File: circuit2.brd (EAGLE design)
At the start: 85.1 x 100 mm, 16 parts, among them IC1 ATMEGA328-20P, IC2 786TV

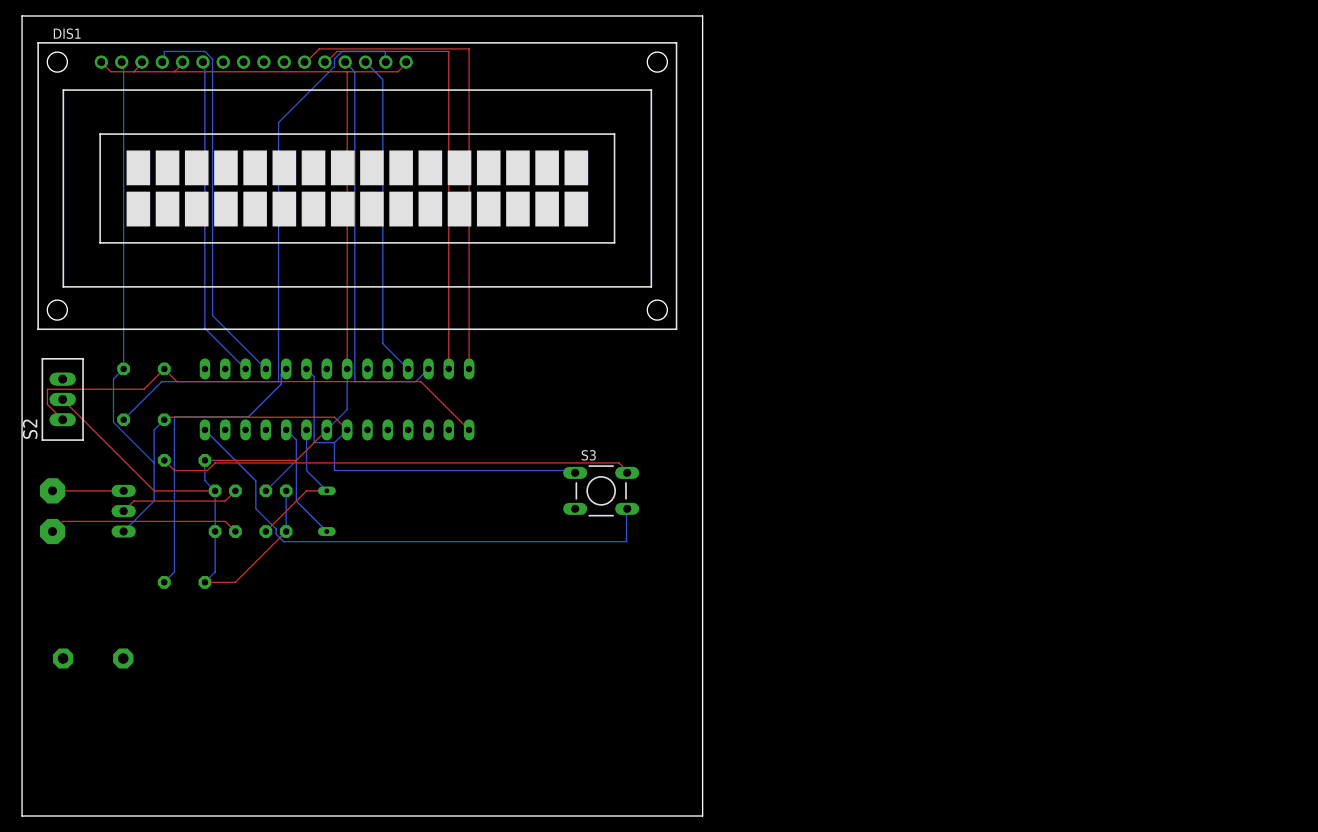
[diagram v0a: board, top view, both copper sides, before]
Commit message: Add files via upload
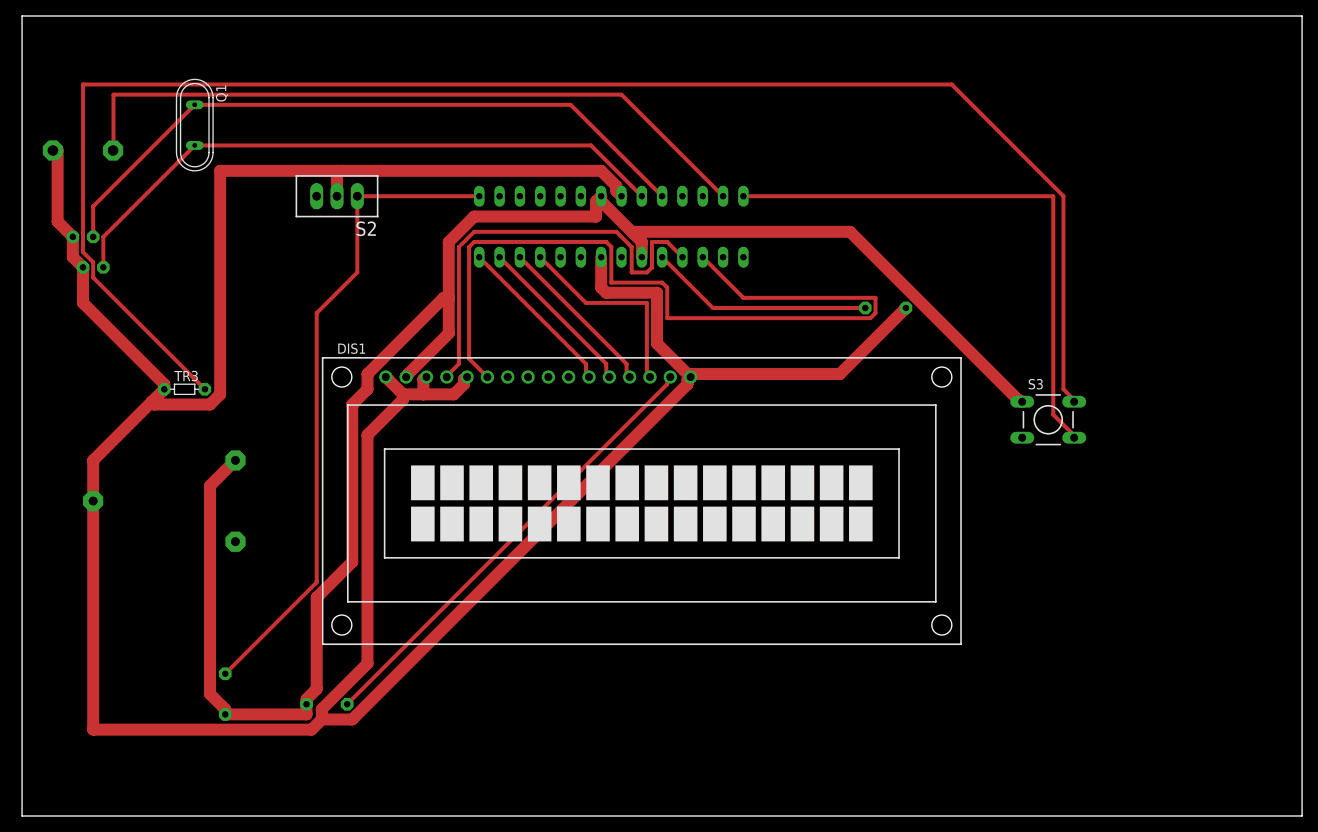
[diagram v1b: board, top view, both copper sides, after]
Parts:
- removed C3: (no value), capacitor-wima:C2.5-2
- removed C4: 10u, capacitor-wima:C2.5-2
- removed IC2: 786TV, linear:TO220V
- G1: value AB9V -> CR2430H; device battery:AB9V -> battery:CR2430H
- moved TR2 94.1 mm to (108.0, 63.5)
- moved SG1 80.0 mm to (7.62, 91.4), turned to 0 degrees
- moved S3 56.6 mm to (128.3, 49.5)
- moved DIS1 53.1 mm to (77.5, 39.4)
- moved Q1 51.0 mm to (21.6, 86.4), flipped to the top, turned to 270 degrees
- moved S2 42.7 mm to (39.4, 77.5), turned to 180 degrees
- moved TR4 42.3 mm to (38.1, 14.0), turned to 0 degrees
- moved TR1 41.9 mm to (25.4, 15.2), turned to 270 degrees
- moved IC1 40.5 mm to (73.7, 73.7), turned to 180 degrees
- moved C2 40.2 mm to (8.89, 68.6), turned to 180 degrees
- moved C1 39.9 mm to (7.62, 72.4), turned to 180 degrees
- moved G1 10.2 mm to (14.0, 39.4), turned to 90 degrees
- moved TR3 8.89 mm to (20.3, 53.3), flipped to the top
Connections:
- removed net N$2: C4.1, IC2.2
- removed net N$3: C3.1, G1.-
- new net N$16: IC1.16
- net GND: now also G1.-, SG1.2; no longer C3.2, C4.2
- net N$1: now also IC1.13, SG1.1; no longer G1.+, IC2.1
- net VCC: now also G1.+; no longer IC2.3
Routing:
- net GND: track 163.0 -> 381.0 mm
- net N$17: track 59.4 -> 199.0 mm
- net N$1: track 8.89 -> 88.5 mm
- net VCC: track 140.7 -> 212.5 mm
- net N$5: track 20.2 -> 84.9 mm
- net N$10: track 40.6 -> 102.9 mm
- net N$6: track 18.4 -> 78.5 mm
- net N$11: track 61.2 -> 20.7 mm
- net N$12: track 55.7 -> 20.7 mm
- net N$13: track 50.3 -> 20.7 mm
- net N$3: track 23.9 -> 0.00 mm
- net N$4: track 61.5 -> 81.8 mm
- net N$15: track 40.6 -> 25.1 mm
- net N$2: track 15.0 -> 0.00 mm
- net N$8: track 72.7 -> 57.7 mm
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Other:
- board size 85.1 x 100 mm -> 160 x 100 mm
